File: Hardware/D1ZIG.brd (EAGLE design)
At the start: 33.6 x 25.4 mm, 5 parts

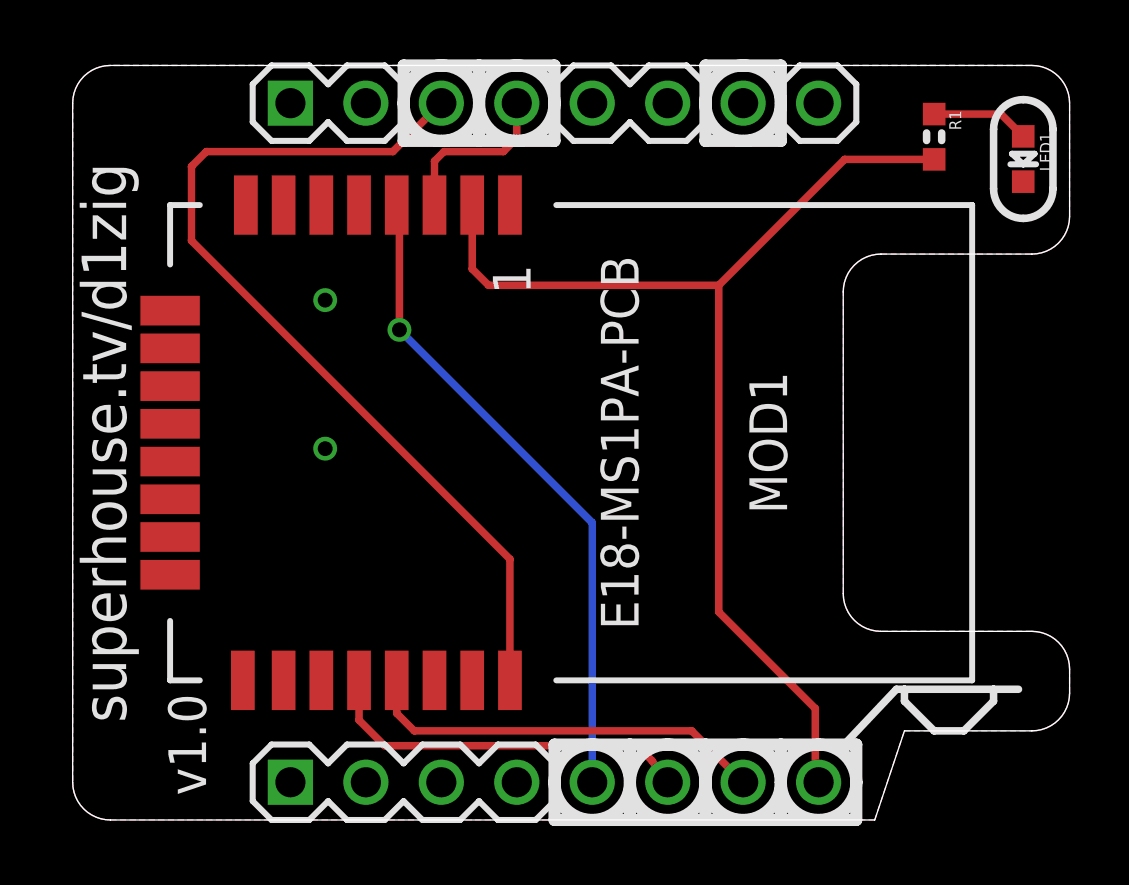
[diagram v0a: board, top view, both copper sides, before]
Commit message: Final DRC and tweaks for v1.0 release
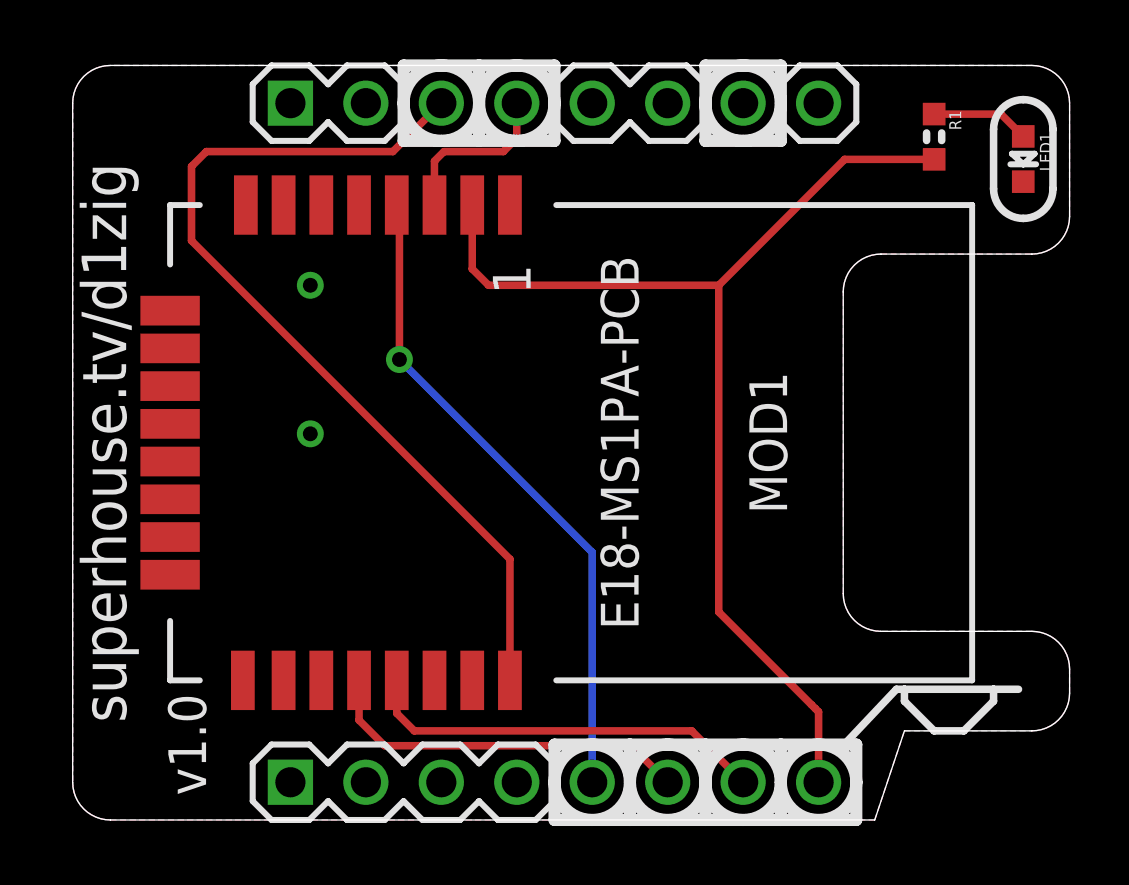
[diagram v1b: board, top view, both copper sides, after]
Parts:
- renumbered J3 to J1, J4 to J2
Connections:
- removed net RX: J2.2
- removed net TX: J2.1
